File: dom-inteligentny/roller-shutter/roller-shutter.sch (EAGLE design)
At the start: 31 parts, among them K1 RP421110, K4 RP421110, Q1 16MHz, T1 BC847, T2 BC847, U1 ATMEGA328, X2 JST-XH-05-PIN-LONG-PAD, X3 JST-XH-05-PIN-LONG-PAD

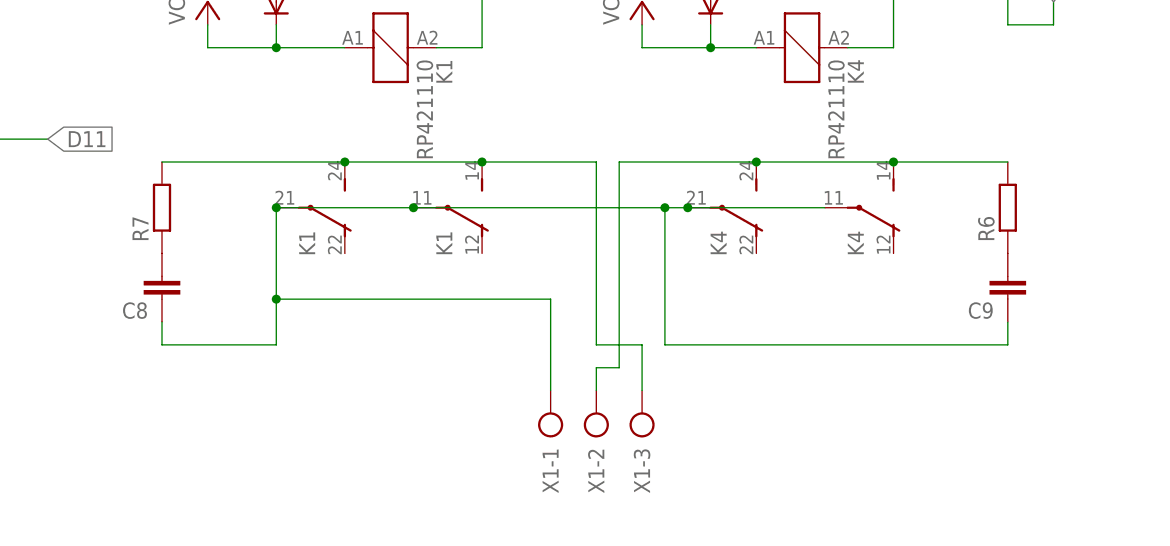
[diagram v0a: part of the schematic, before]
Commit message: Roller shutter ark change
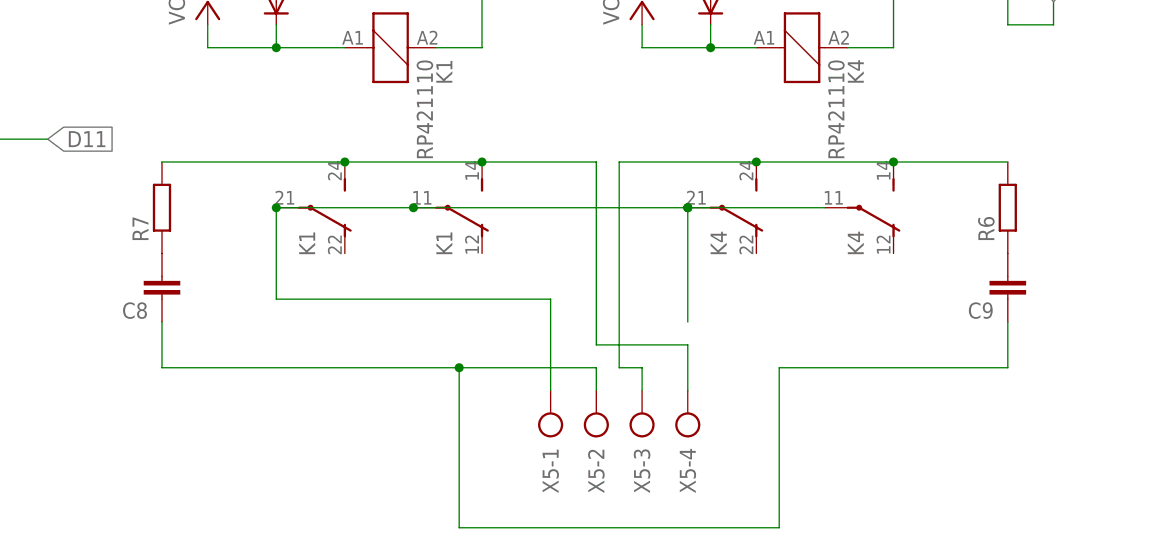
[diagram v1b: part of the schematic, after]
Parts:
- removed X1: (no value), con-ptr500:AK500/3
- added X5: (no value), con-ptr500:AK500/4
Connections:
- new net N$11: C8.1, C9.1, X5-2.KL
- net N$4: now also X5-1.KL; no longer C8.1, C9.1, X1-1.KL
- net N$7: now also X5-4.KL; no longer X1-3.KL
- net N$8: now also X5-3.KL; no longer X1-2.KL
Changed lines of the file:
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@@
 <part name="JP2" library="pinhead" library_urn="urn:adsk.eagle:library:325" deviceset="PINHD-1X3" device="" package3d_urn="urn:adsk.eagle:package:22458/2"/>
 <part name="X4" library="con-ptr500" library_urn="urn:adsk.eagle:library:181" deviceset="AK500/3" device="" package3d_urn="urn:adsk.eagle:package:9883/1"/>
-<part name="X1" library="con-ptr500" library_urn="urn:adsk.eagle:library:181" deviceset="AK500/3" device="" package3d_urn="urn:adsk.eagle:package:9883/1"/>
 <part name="GND9" library="supply1" library_urn="urn:adsk.eagle:library:371" deviceset="GND" device=""/>
 <part name="P+8" library="supply1" library_urn="urn:adsk.eagle:library:371" deviceset="VCC" device=""/>
 <part name="JP6" library="pinhead-zmiany-JP" deviceset="PINHD-3X4" device=""/>
+<part name="X5" library="con-ptr500" library_urn="urn:adsk.eagle:library:181" deviceset="AK500/4" device="" package3d_urn="urn:adsk.eagle:package:9887/1"/>
 </parts>
 <sheets>
@@
 <attribute name="VALUE" x="334.01" y="171.577" size="1.778" layer="96" rot="MR0"/>
 </instance>
-<instance part="X1" gate="-1" x="294.64" y="43.18" smashed="yes" rot="R90">
-<attribute name="NAME" x="293.751" y="41.91" size="1.778" layer="95" rot="R270"/>
-</instance>
-<instance part="X1" gate="-2" x="299.72" y="43.18" smashed="yes" rot="R90">
-<attribute name="NAME" x="298.831" y="41.91" size="1.778" layer="95" rot="R270"/>
-</instance>
-<instance part="X1" gate="-3" x="304.8" y="43.18" smashed="yes" rot="R90">
-<attribute name="NAME" x="303.911" y="41.91" size="1.778" layer="95" rot="R270"/>
-<attribute name="VALUE" x="308.483" y="39.37" size="1.778" layer="96" rot="R90"/>
-</instance>
 <instance part="GND9" gate="1" x="358.14" y="119.38" smashed="yes">
 <attribute name="VALUE" x="355.6" y="116.84" size="1.778" layer="96"/>
@@
 <attribute name="NAME" x="339.09" y="168.275" size="1.778" layer="95"/>
 <attribute name="VALUE" x="339.09" y="152.4" size="1.778" layer="96"/>
+</instance>
+<instance part="X5" gate="-1" x="294.64" y="43.18" smashed="yes" rot="R90">
+<attribute name="NAME" x="293.751" y="41.91" size="1.778" layer="95" rot="R270"/>
+</instance>
+<instance part="X5" gate="-2" x="299.72" y="43.18" smashed="yes" rot="R90">
+<attribute name="NAME" x="298.831" y="41.91" size="1.778" layer="95" rot="R270"/>
+</instance>
+<instance part="X5" gate="-3" x="304.8" y="43.18" smashed="yes" rot="R90">
+<attribute name="NAME" x="303.911" y="41.91" size="1.778" layer="95" rot="R270"/>
+</instance>
+<instance part="X5" gate="-4" x="309.88" y="43.18" smashed="yes" rot="R90">
+<attribute name="NAME" x="308.991" y="41.91" size="1.778" layer="95" rot="R270"/>
+<attribute name="VALUE" x="313.563" y="39.37" size="1.778" layer="96" rot="R90"/>
 </instance>
 </instances>
@@
 <pinref part="K1" gate="3" pin="P"/>
 <wire x1="279.4" y1="68.58" x2="264.16" y2="68.58" width="0.1524" layer="91"/>
-<wire x1="309.88" y1="68.58" x2="307.34" y2="68.58" width="0.1524" layer="91"/>
 <junction x="309.88" y="68.58"/>
 <junction x="279.4" y="68.58"/>
-<wire x1="307.34" y1="68.58" x2="279.4" y2="68.58" width="0.1524" layer="91"/>
+<wire x1="309.88" y1="68.58" x2="279.4" y2="68.58" width="0.1524" layer="91"/>
 <wire x1="264.16" y1="68.58" x2="264.16" y2="58.42" width="0.1524" layer="91"/>
 <junction x="264.16" y="68.58"/>
 <wire x1="264.16" y1="58.42" x2="294.64" y2="58.42" width="0.1524" layer="91"/>
-<pinref part="C8" gate="G$1" pin="1"/>
-<wire x1="251.46" y1="55.88" x2="251.46" y2="53.34" width="0.1524" layer="91"/>
-<wire x1="251.46" y1="53.34" x2="264.16" y2="53.34" width="0.1524" layer="91"/>
-<wire x1="264.16" y1="53.34" x2="264.16" y2="58.42" width="0.1524" layer="91"/>
-<junction x="264.16" y="58.42"/>
-<pinref part="C9" gate="G$1" pin="1"/>
-<wire x1="345.44" y1="55.88" x2="345.44" y2="53.34" width="0.1524" layer="91"/>
-<wire x1="345.44" y1="53.34" x2="307.34" y2="53.34" width="0.1524" layer="91"/>
-<wire x1="307.34" y1="53.34" x2="307.34" y2="68.58" width="0.1524" layer="91"/>
-<junction x="307.34" y="68.58"/>
-<pinref part="X1" gate="-1" pin="KL"/>
+<wire x1="309.88" y1="55.88" x2="309.88" y2="68.58" width="0.1524" layer="91"/>
+<junction x="309.88" y="68.58"/>
 <wire x1="294.64" y1="48.26" x2="294.64" y2="58.42" width="0.1524" layer="91"/>
+<pinref part="X5" gate="-1" pin="KL"/>
 </segment>
 </net>
@@
 <junction x="287.02" y="73.66"/>
 <wire x1="299.72" y1="73.66" x2="299.72" y2="53.34" width="0.1524" layer="91"/>
+<wire x1="299.72" y1="53.34" x2="309.88" y2="53.34" width="0.1524" layer="91"/>
+<pinref part="X5" gate="-4" pin="KL"/>
+<wire x1="309.88" y1="53.34" x2="309.88" y2="48.26" width="0.1524" layer="91"/>
 <pinref part="R7" gate="G$1" pin="2"/>
-<wire x1="251.46" y1="73.66" x2="271.78" y2="73.66" width="0.1524" layer="91"/>
+<wire x1="271.78" y1="73.66" x2="251.46" y2="73.66" width="0.1524" layer="91"/>
 <junction x="271.78" y="73.66"/>
-<wire x1="299.72" y1="53.34" x2="304.8" y2="53.34" width="0.1524" layer="91"/>
-<pinref part="X1" gate="-3" pin="KL"/>
-<wire x1="304.8" y1="53.34" x2="304.8" y2="48.26" width="0.1524" layer="91"/>
 </segment>
 </net>
@@
 <junction x="317.5" y="73.66"/>
 <wire x1="302.26" y1="73.66" x2="302.26" y2="50.8" width="0.1524" layer="91"/>
+<wire x1="302.26" y1="50.8" x2="304.8" y2="50.8" width="0.1524" layer="91"/>
+<pinref part="X5" gate="-3" pin="KL"/>
+<wire x1="304.8" y1="50.8" x2="304.8" y2="48.26" width="0.1524" layer="91"/>
 <pinref part="R6" gate="G$1" pin="2"/>
-<wire x1="332.74" y1="73.66" x2="345.44" y2="73.66" width="0.1524" layer="91"/>
+<wire x1="345.44" y1="73.66" x2="332.74" y2="73.66" width="0.1524" layer="91"/>
 <junction x="332.74" y="73.66"/>
-<wire x1="302.26" y1="50.8" x2="299.72" y2="50.8" width="0.1524" layer="91"/>
-<pinref part="X1" gate="-2" pin="KL"/>
-<wire x1="299.72" y1="50.8" x2="299.72" y2="48.26" width="0.1524" layer="91"/>
 </segment>
 </net>
@@
 </segment>
 </net>
+<net name="N$11" class="0">
+<segment>
+<pinref part="C8" gate="G$1" pin="1"/>
+<wire x1="251.46" y1="55.88" x2="251.46" y2="50.8" width="0.1524" layer="91"/>
+<pinref part="X5" gate="-2" pin="KL"/>
+<wire x1="299.72" y1="48.26" x2="299.72" y2="50.8" width="0.1524" layer="91"/>
+<wire x1="299.72" y1="50.8" x2="284.48" y2="50.8" width="0.1524" layer="91"/>
+<wire x1="284.48" y1="50.8" x2="284.48" y2="33.02" width="0.1524" layer="91"/>
+<wire x1="284.48" y1="33.02" x2="320.04" y2="33.02" width="0.1524" layer="91"/>
+<wire x1="320.04" y1="33.02" x2="320.04" y2="50.8" width="0.1524" layer="91"/>
+<wire x1="251.46" y1="50.8" x2="284.48" y2="50.8" width="0.1524" layer="91"/>
+<junction x="284.48" y="50.8"/>
+<wire x1="320.04" y1="50.8" x2="345.44" y2="50.8" width="0.1524" layer="91"/>
+<pinref part="C9" gate="G$1" pin="1"/>
+<wire x1="345.44" y1="50.8" x2="345.44" y2="55.88" width="0.1524" layer="91"/>
+</segment>
+</net>
